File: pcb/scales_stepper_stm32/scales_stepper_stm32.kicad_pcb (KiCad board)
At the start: 2 copper layers, 15 parts, among them J3 Screw_Terminal_01x02, J4 Screw_Terminal_01x04, U1 BP, U2 LM78M05_TO252

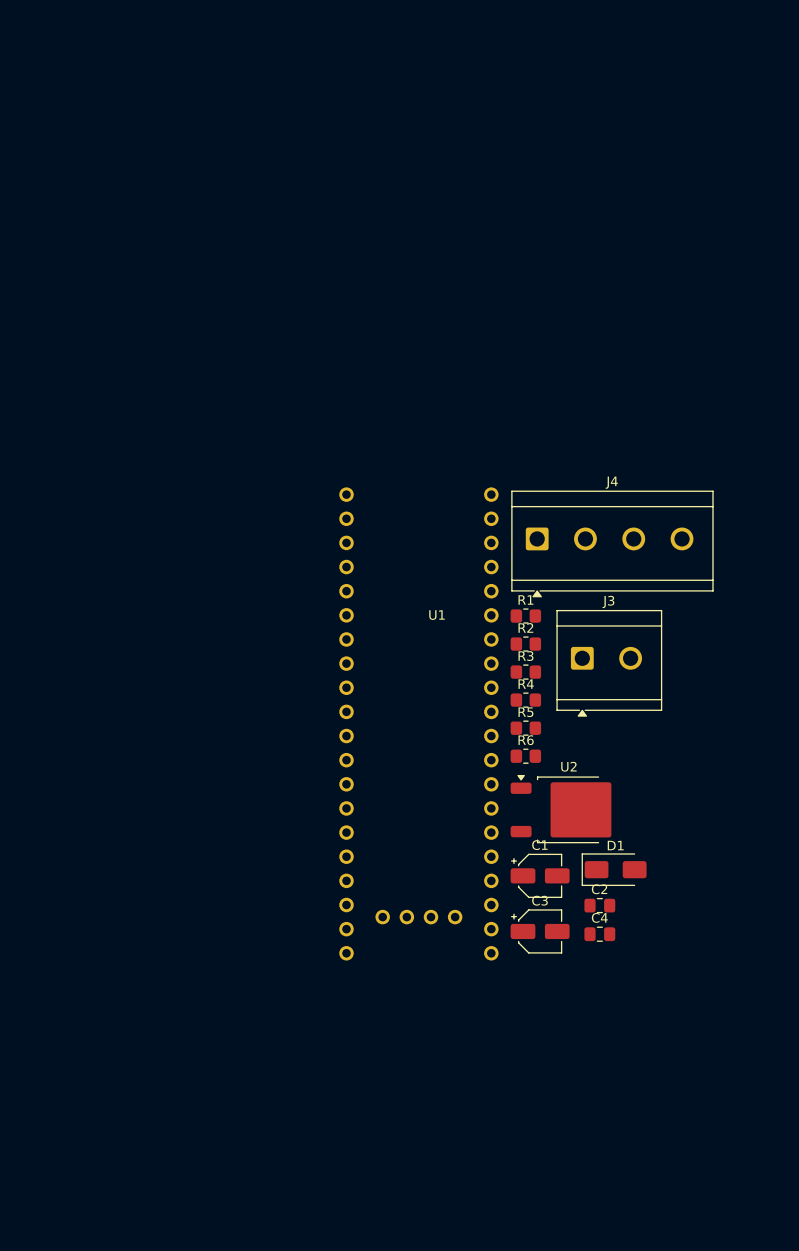
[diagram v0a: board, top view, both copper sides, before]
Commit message: morse code
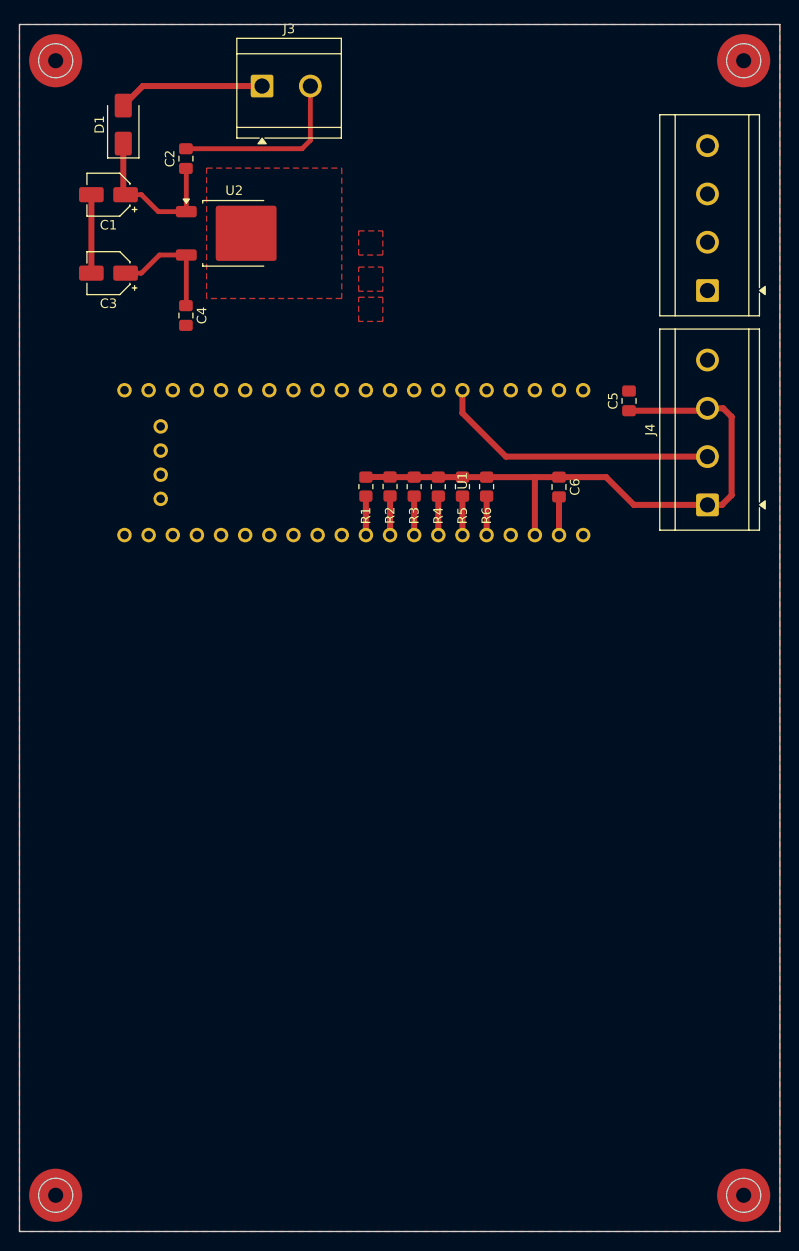
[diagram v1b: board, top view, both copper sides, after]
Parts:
- added C5: 100n, Capacitor_SMD:C_0805_2012Metric_Pad1.18x1.45mm_HandSolder, F.Cu at (153.0, 57.4)
- added C6: 100n, Capacitor_SMD:C_0805_2012Metric_Pad1.18x1.45mm_HandSolder, F.Cu at (145.7, 66.4)
- added J5: Screw_Terminal_01x04, TerminalBlock_CUI:TerminalBlock_CUI_TB007-508-04_1x04_P5.08mm_Horizontal, F.Cu at (161.3, 45.8)
- moved D1 94.0 mm to (99.8, 28.3), turned to 90 degrees
- moved C2 89.9 mm to (106.4, 31.9), turned to 90 degrees
- moved C1 84.9 mm to (98.3, 35.7), turned to 180 degrees
- moved C3 82.8 mm to (98.3, 43.9), turned to 180 degrees
- moved C4 78.3 mm to (106.4, 48.4), turned to -90 degrees
- moved U2 70.2 mm to (111.5, 39.8)
- moved J3 69.0 mm to (114.4, 24.3)
- moved R6 28.7 mm to (138.0, 66.4), turned to -90 degrees
- moved R5 26.3 mm to (135.5, 66.4), turned to -90 degrees
- moved R4 24.3 mm to (133.0, 66.4), turned to -90 degrees
- moved U1 23.1 mm to (127.3, 65.8), turned to -90 degrees
- moved R3 22.8 mm to (130.4, 66.4), turned to -90 degrees
- moved R2 21.9 mm to (127.9, 66.4), turned to -90 degrees
- moved R1 21.7 mm to (125.3, 66.4), turned to -90 degrees
- moved J4 18.3 mm to (161.3, 68.3), turned to 90 degrees
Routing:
- net +3V3: track 0.00 -> 65.7 mm
- net GND: track 0.00 -> 31.5 mm
- net DIR: track 0.00 -> 30.1 mm
- net Net-(D1-K): track 0.00 -> 17.2 mm
- net +24V: track 0.00 -> 15.5 mm
- net +5V: track 0.00 -> 12.5 mm
- net BUTT_JOGR: track 0.00 -> 4.11 mm
- net ES_R: track 0.00 -> 4.10 mm
- net ES_L: track 0.00 -> 4.10 mm
- net BUTT_STEPR: track 0.00 -> 4.10 mm
- net BUTT_STEPL: track 0.00 -> 4.10 mm
- net BUTT_JOGL: track 0.00 -> 4.10 mm
- added copper zone on F.Cu, net GND
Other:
- board outline added: 80 x 127 mm
